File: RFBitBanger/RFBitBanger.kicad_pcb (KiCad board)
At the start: 2 copper layers, 149 x 88 mm, 222 parts, among them J1 POWER, J10 Conn_01x04, J11 SPEAKER, J12 Conn_Coaxial, J13 Conn_01x01, J2 Barrel_Jack, J3 Conn_01x01, J4 Conn_01x01, J5 Conn_01x04, J6 Conn_01x01, J7 Conn_01x01, J8 Conn_01x01, J9 ICSP, P1 Mini-DIN_6pins_ver4, Q1 2N3904, Q10 2N3904, Q11 2N3904, Q12 2N3904, Q13 2N2907, Q14 2N3904, Q2 2N3904, Q3 2N3904, Q4 2N3904, Q5 2N3904, Q6 2N3904, Q7 2N3904, Q8 2N2907, Q9 2N3904, SW1 SW_Push, SW2 SW_Push, SW3 SW_Push, SW4 SW_Push, SW5 SW_Push, T1 Trifilar, T2 Trifilar, T3 Current, T4 Common-Mode Choke, U1 ATMEGA328-PU, U2 LM7805_TO220, U3 LM386, U4 LM358, U5 LCD-016N002L, U6 SI5351A, Y1 16 MHz, Y2 7.X MHz, Y3 27 MHz, Y4 7.X MHz, Y5 7.X MHz

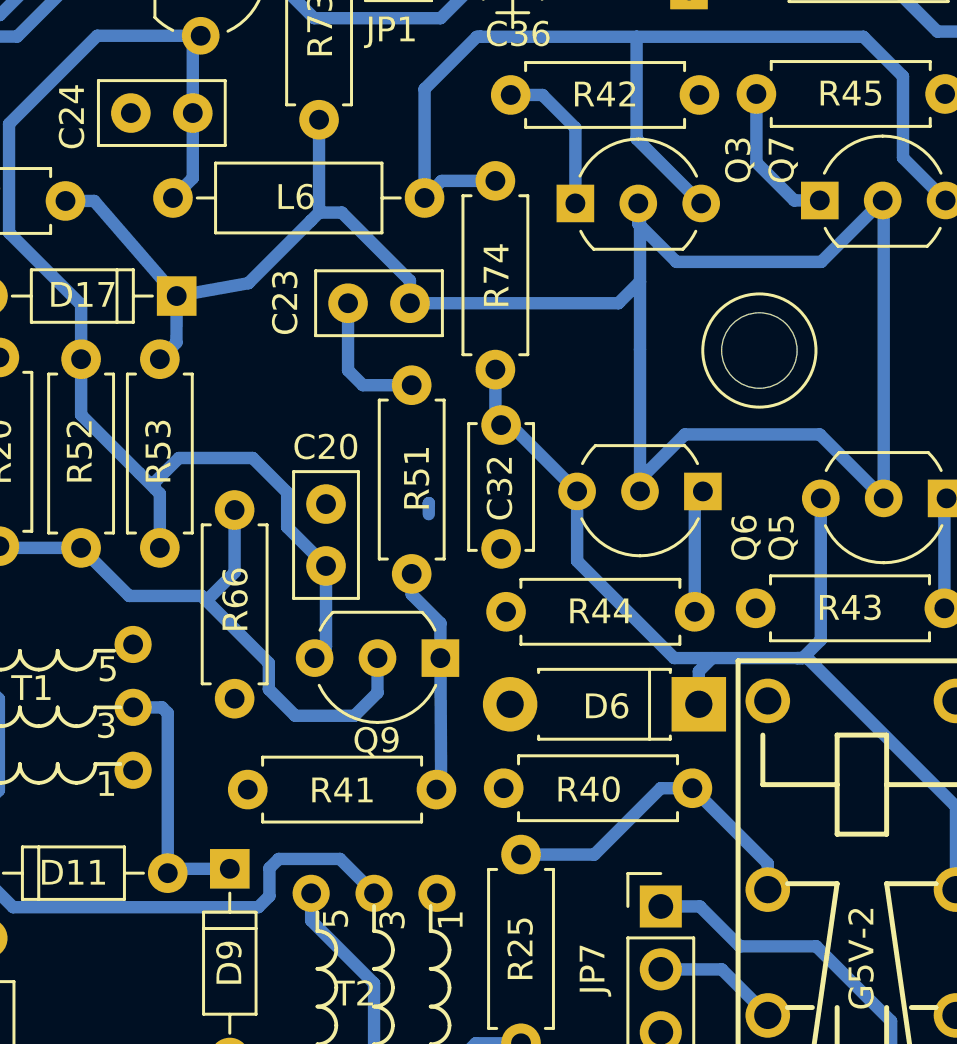
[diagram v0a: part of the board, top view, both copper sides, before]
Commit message: Added README.md
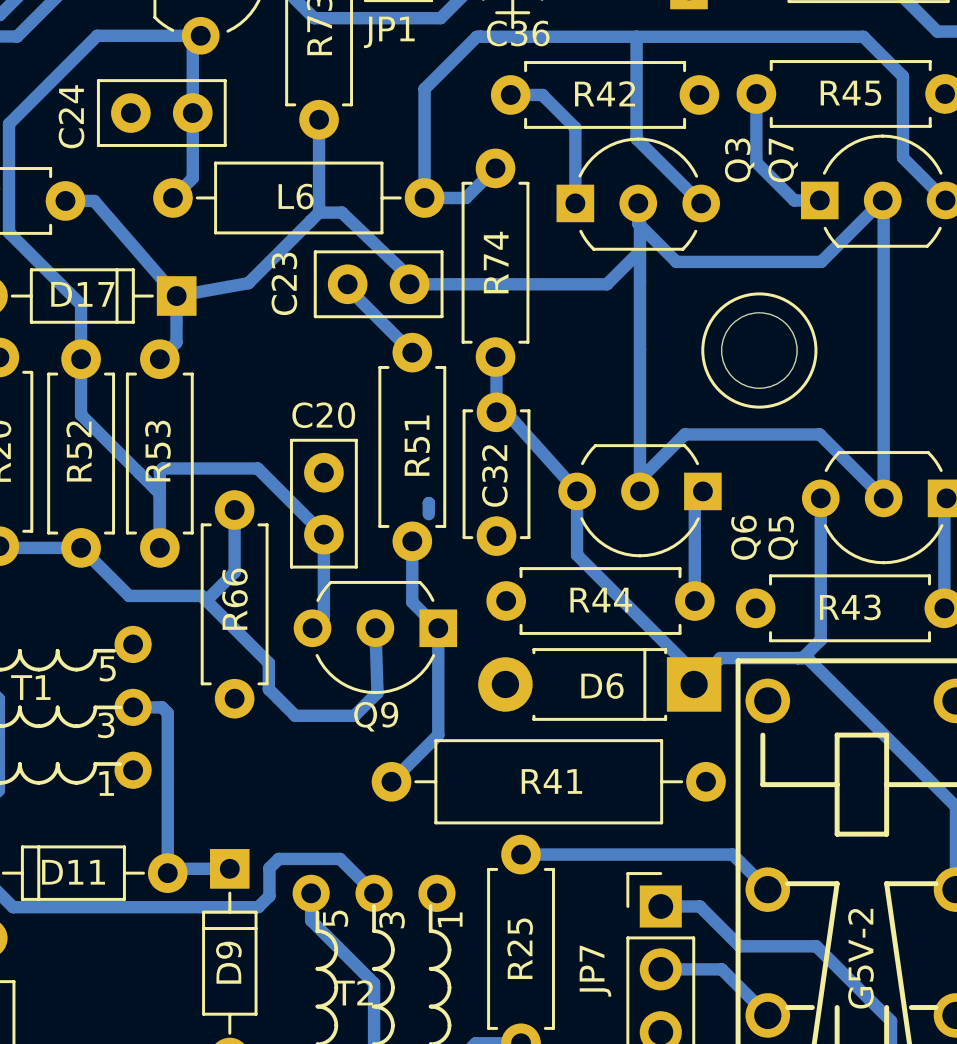
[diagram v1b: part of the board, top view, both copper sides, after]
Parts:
- removed R40: NC, Resistors_THT:R_Axial_DIN0207_L6.3mm_D2.5mm_P7.62mm_Horizontal
- R41: footprint Resistors_THT:R_Axial_DIN0207_L6.3mm_D2.5mm_P7.62mm_Horizontal -> Resistors_THT:R_Axial_DIN0309_L9.0mm_D3.2mm_P12.70mm_Horizontal
- moved R41 18.5 mm to (177.7, 102.1), turned to 180 degrees
- moved R51 1.32 mm to (165.8, 92.4)
- moved C20 1.27 mm to (162.2, 89.6)
- moved Q9 1.21 mm to (166.9, 95.9)
- moved D6 0.82 mm to (177.2, 98.2)
- moved C23 0.77 mm to (163.2, 82.0)
- moved C32 0.55 mm to (169.2, 87.2)
- moved R74 0.51 mm to (169.2, 77.3)
- moved R44 0.44 mm to (177.2, 94.8)
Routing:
- net RF: track 13.4 -> 10.6 mm
- net Net-(Q9-Pad1): track 9.27 -> 11.1 mm
- net Net-(C23-Pad1): track 5.53 -> 3.84 mm
- net Net-(C20-Pad2): track 51.4 -> 52.7 mm
- net Net-(Q9-Pad2): track 24.6 -> 25.9 mm
- net Net-(C23-Pad2): track 83.9 -> 83.4 mm
